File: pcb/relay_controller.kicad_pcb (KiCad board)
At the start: 2 copper layers, 118.1 x 55.1 mm, 46 parts, among them P1 PWR_JACK_2.5x5.5, P2 HEADER_01X03_SMD_RA, P3 HEADER_01X03_SMD_RA, P4 HEADER_01X03_SMD_RA, P5 HEADER_01X03_SMD_RA, P6 HEADER_01X02_SMD_RA, P7 BNC_DOUBLE_RA, SW1 SPST_SLIDE_AS, T1 TERM_BLK_ANG_2_PIN, T2 TERM_BLK_ANG_2_PIN, T3 TERM_BLK_ANG_2_PIN, T4 TERM_BLK_ANG_2_PIN, T5 TERM_BLK_ANG_2_PIN, T6 TERM_BLK_ANG_2_PIN, T7 TERM_BLK_ANG_2_PIN, T8 TERM_BLK_ANG_2_PIN, U1 SSR_DC_6PIN, U2 SSR_DC_6PIN, U3 SSR_DC_6PIN, U4 SSR_DC_6PIN, U5 SSR_DC_6PIN, U6 SSR_DC_6PIN, U7 SSR_DC_6PIN, U8 SSR_DC_6PIN

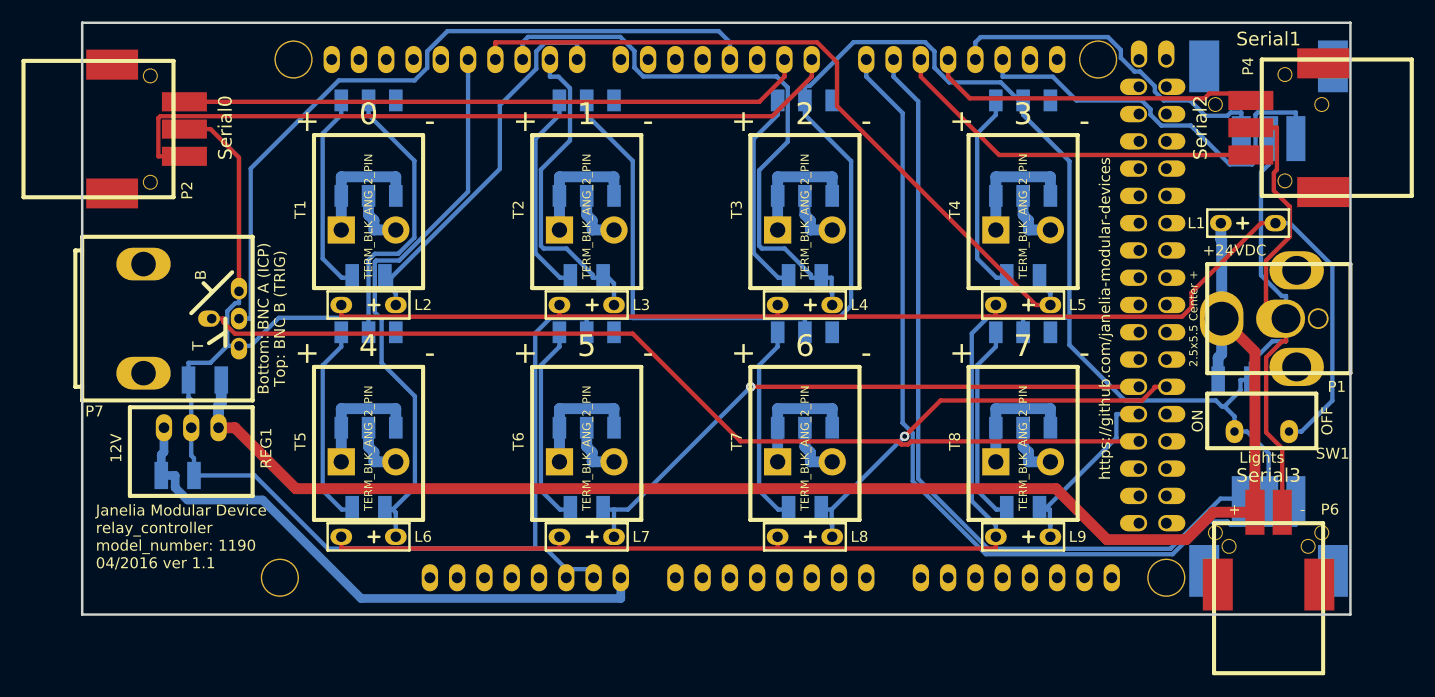
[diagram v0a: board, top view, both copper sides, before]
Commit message: Removed traces.
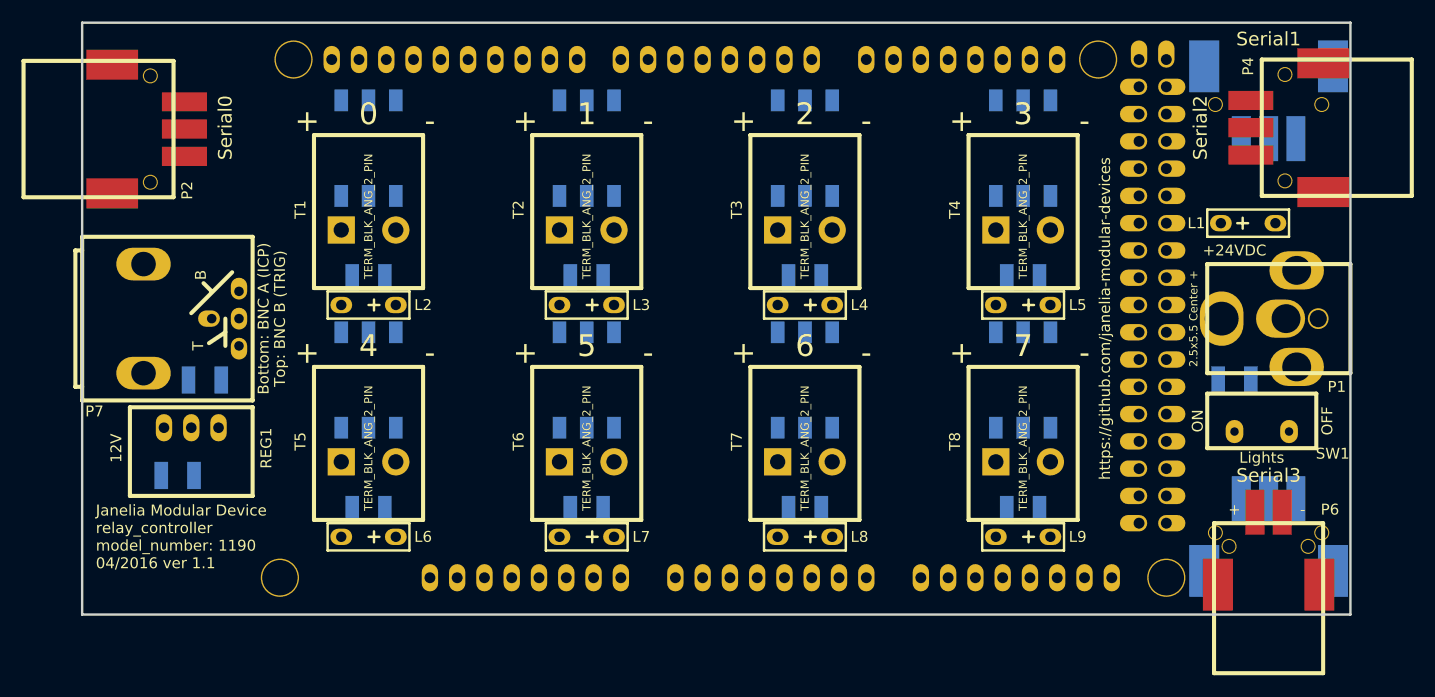
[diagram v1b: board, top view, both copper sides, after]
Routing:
- net GND: track 375.8 -> 0.00 mm
- net /LED_GND: track 209.7 -> 0.00 mm
- net VAA: track 140.5 -> 0.00 mm
- net /BNC_A: track 91.5 -> 0.00 mm
- net /TX3: track 83.4 -> 0.00 mm
- net /RX3: track 74.7 -> 0.00 mm
- net /RX0: track 70.0 -> 0.00 mm
- net /RELAY_3: track 68.9 -> 0.00 mm
- net /BNC_B: track 67.9 -> 0.00 mm
- net /TX0: track 58.4 -> 0.00 mm
- net /RELAY_5: track 57.2 -> 0.00 mm, vias 1 -> 0
- net /RELAY_2: track 55.9 -> 0.00 mm
- net /V_IN: track 54.7 -> 0.00 mm
- net /RELAY_4: track 52.6 -> 0.00 mm
- net /RX1: track 39.5 -> 0.00 mm
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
